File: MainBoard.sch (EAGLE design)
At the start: 37 parts, among them U1 LM1085IT-3.3/NOPBT03BM, U2 LM1085IT-5.0/NOPB

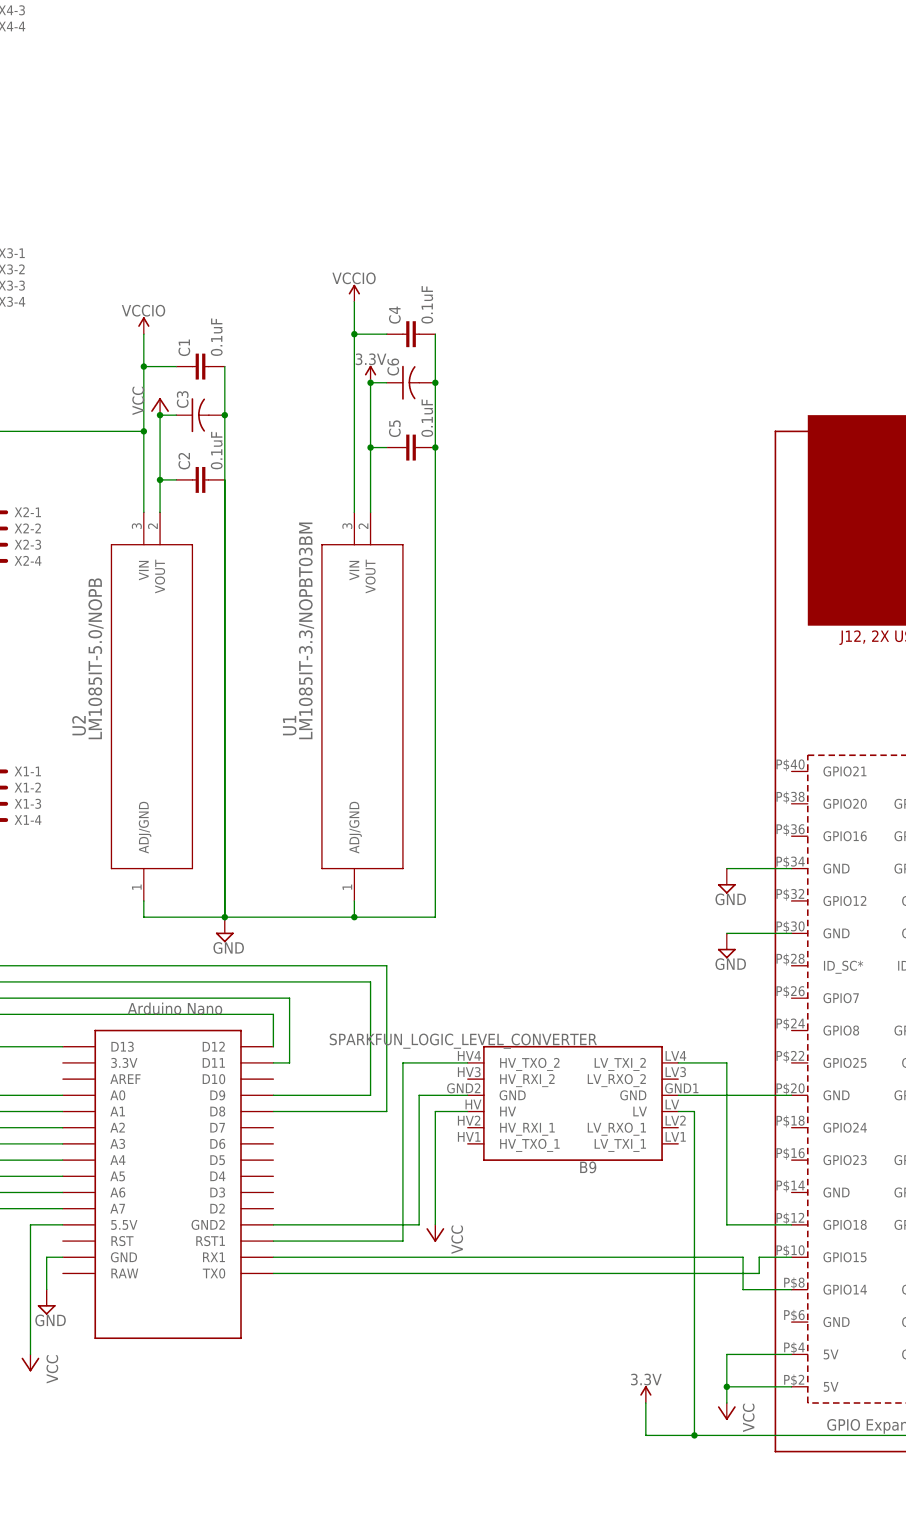
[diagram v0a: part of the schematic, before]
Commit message: Added Pi Power Dictatorship
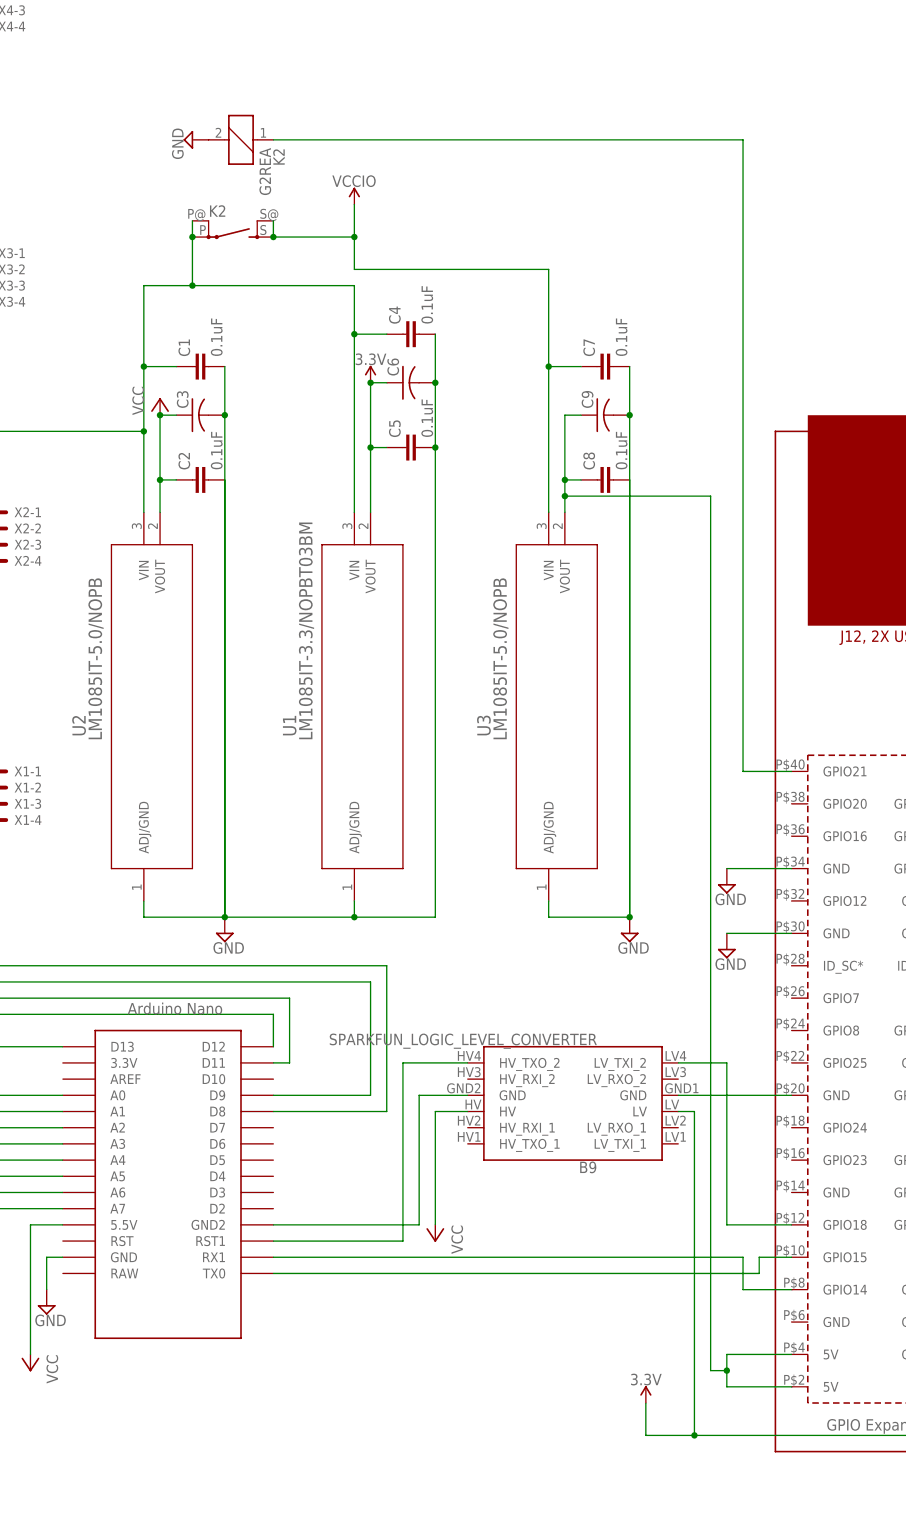
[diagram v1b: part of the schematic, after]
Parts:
- added C7, C8: 0.1uF, SparkFun-Capacitors:0.1UF-KIT-EZ-50V-20%
- added C9: (no value), rcl:C-US025-050X050
- added K2: G2REA, relay:G2REA
- added U3: LM1085IT-5.0/NOPB, LM1085:LM1085IT-5.0/NOPB
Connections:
- new net N$39: C8.1, C9.1, PCB1.5V@2, PCB1.5V@4, U3.VOUT
- new net N$61: B1.VM, B2.VM, B3.VM, B4.VM, B5.VM, B6.VM, B7.VM, B8.VM, C1.1, C4.1, K22.P, K22.P@1, U2.VIN
- new net N$62: K21.1, PCB1.GPIO21
- net GND: now also C7.2, C8.2, C9.2, K21.2, U3.ADJ/GND
- net VCC: no longer PCB1.5V@2, PCB1.5V@4
- net VCCIO: now also C7.1, K22.S, K22.S@1, U3.VIN; no longer B1.VM, B2.VM, B3.VM, B4.VM, B5.VM, B6.VM, B7.VM, B8.VM, C1.1, C4.1, U2.VIN
